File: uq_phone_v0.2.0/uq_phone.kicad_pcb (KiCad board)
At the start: 6 copper layers, 118.2 x 108 mm, 195 parts, among them J1 PJ-242C, J2 124018312112A, J3 BM03B-ACHSS-GAN-TF_LF__SN_, J4 20279-001E-03, J5 20279-001E-03, J6 Conn_ARM_SWD_TagConnect_TC2030, J8 MCS-302S-C1, M1 C08-00A, Q1 MMBT3904LP-7, Q2 MMBT3904LP-7, SW1 SKTAAAE010, SW10 SKTAAAE010, SW11 SKTAAAE010, SW12 SKTAAAE010, SW13 SKTAAAE010, SW14 SKTAAAE010, SW15 SKTAAAE010, SW16 SKSCLCE010, SW17 SKTAAAE010, SW18 SKTAAAE010, SW19 SKTAAAE010, SW2 SKTAAAE010, SW20 SKTAAAE010, SW21 SKTAAAE010, SW22 SKSCLCE010, SW23 SKTAAAE010, SW24 SKTAAAE010, SW25 SKTAAAE010, SW26 SKTAAAE010, SW27 SKTAAAE010, SW28 SKTAAAE010, SW29 SKTAAAE010, SW3 SKTAAAE010, SW30 SKTAAAE010, SW31 SKTAAAE010, SW32 SKTAAAE010, SW33 SKTAAAE010, SW34 SKTAAAE010, SW35 SKTAAAE010, SW36 SKTAAAE010, SW37 SKTAAAE010, SW38 SKTAAAE010, SW39 SKTAAAE010, SW4 SKTAAAE010, SW40 SKTAAAE010, SW41 SKTAAAE010, SW5 SKTAAAE010, SW6 SKSCLCE010, SW7 SKTAAAE010, SW8 SKTAAAE010, SW9 SKTAAAE010, U1 TPS62162DSGR, U10 TPD8F003DQDR, U11 LSM6DSVTR, U12 DRV2603RUNR, U13 TS3A5018RSVR, U14 NAU88C22YG, U15 TPS22964CYZPR, U2 MCP73871-2CCI_ML, U3 BQ27441DRZR-G1A, U4 WP SNAP-IN BASE_6000636, U5 TXB0108YZPR2, U6 STM32H733VGHx, U7 TXB0108YZPR2, U8 TPD3F303DQDR, U9 MCP1664T-E/OT

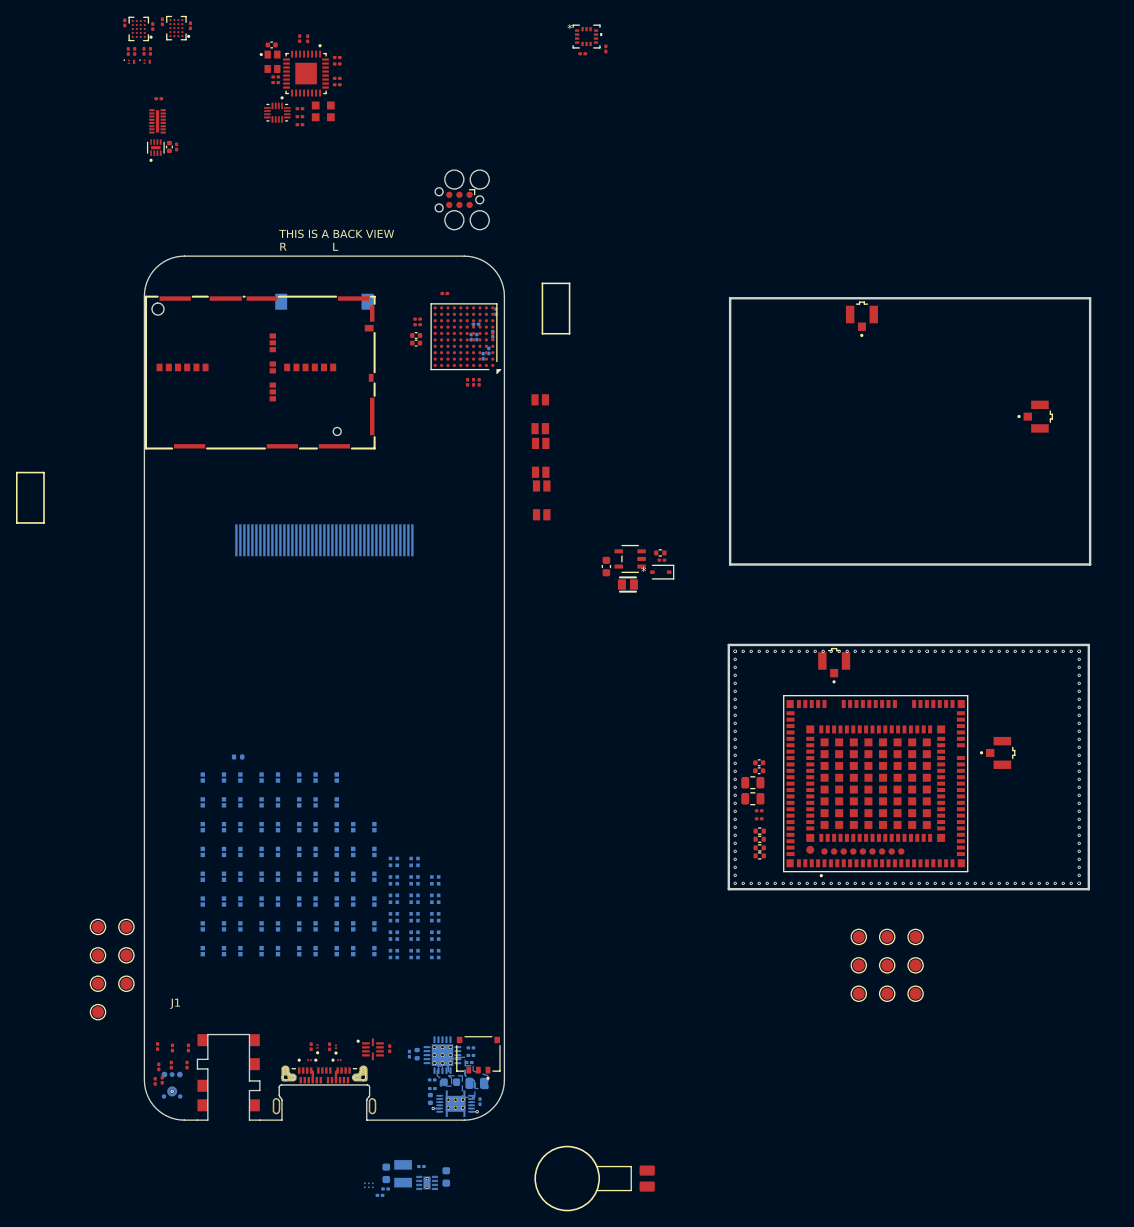
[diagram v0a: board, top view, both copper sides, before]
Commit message: New Layout
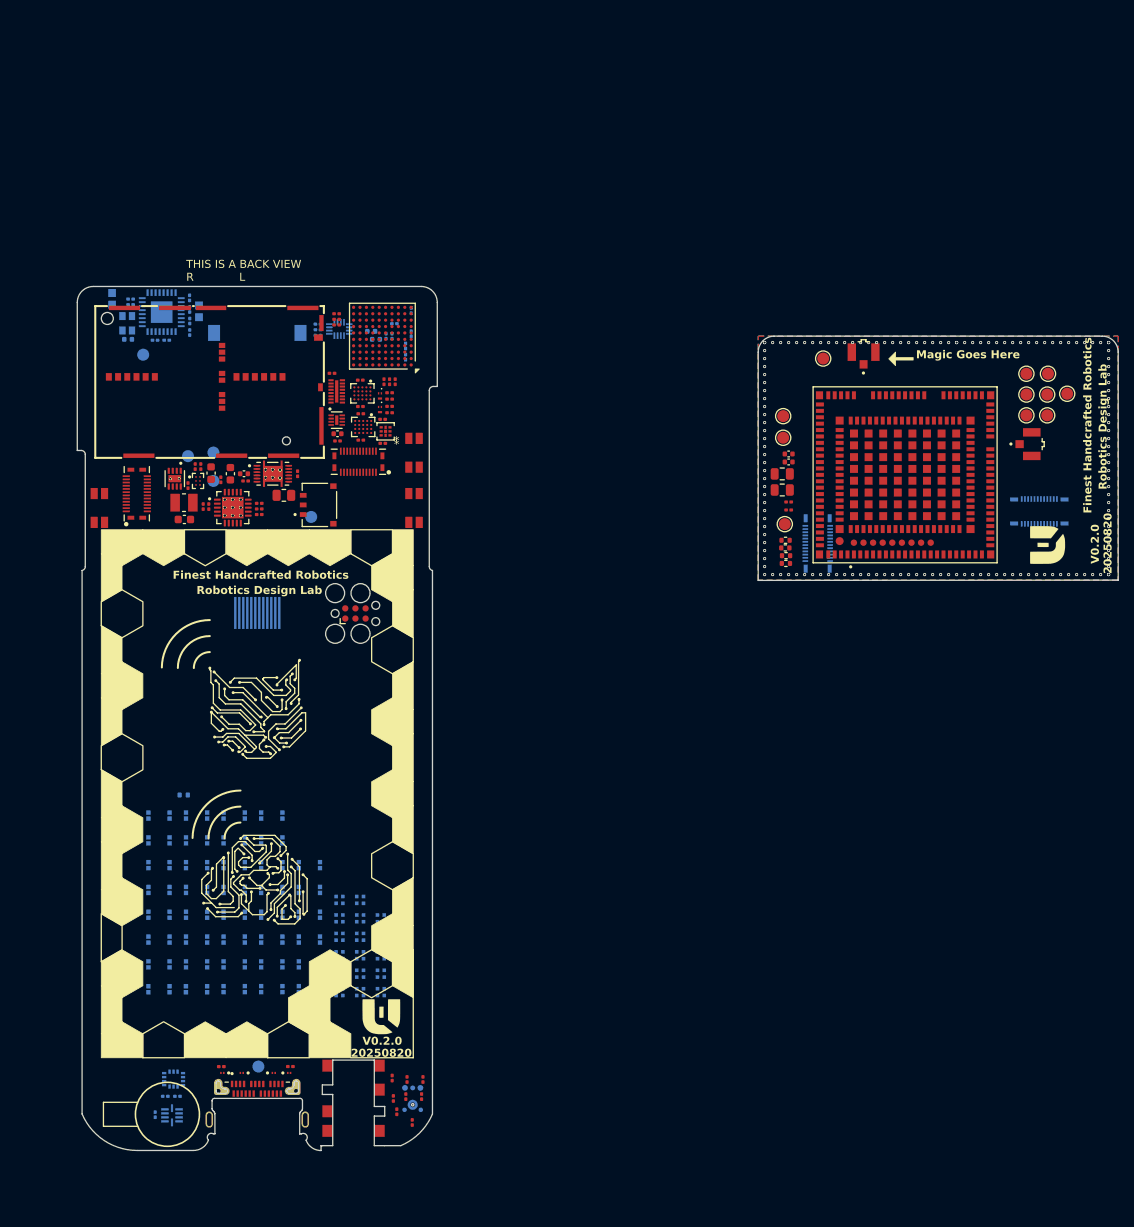
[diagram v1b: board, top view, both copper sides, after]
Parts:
- removed C27: 10uF, Capacitor_SMD:C_0603_1608Metric
- removed C28: 4.7uF, Capacitor_SMD:C_0201_0603Metric
- removed D2: PMEG2010EA, Diode_SMD:D_SOD-323
- removed Disp1: AFR240320A0-2.0INTM, custom_footprints:Display
- removed the J4 at (116.3, 24.4)
- removed the J5 at (138.6, 37.2)
- removed L2: 4.7uH, custom_footprints:IND-SMD_L2.0-W1.2_MTQH201208S4R7MBT
- removed R21: 4.7k, Resistor_SMD:R_0201_0603Metric
- removed R29: 3.83R, Resistor_SMD:R_0402_1005Metric
- removed U9: MCP1664T-E/OT, MCP1664T_E_OT:SOT-23-5_OT_MCH
- added C50: 100nF, Capacitor_SMD:C_0201_0603Metric, F.Cu at (56.4, 37.5)
- added C51: 100nF, Capacitor_SMD:C_0201_0603Metric, F.Cu at (56.5, 40.5)
- added DISP1: HS20HS072RX, custom_footprints:Display, B.Cu at (40.8, 53.9)
- added J10: 513382474, 513382474:CON_513382474, B.Cu at (138.5, 49.0)
- added J11: 513382474, 513382474:CON_513382474, B.Cu at (110.8, 53.0)
- added J7: 559092474, 559092474:CON_559092474, F.Cu at (25.7, 46.8)
- added J9: 559092474, 559092474:CON_559092474, F.Cu at (53.4, 42.8)
- added R4: 4.7k, Resistor_SMD:R_0201_0603Metric, F.Cu at (58.0, 32.8)
- added REF**: Art_large, custom_footprints:Art_large, F.Cu at (40.8, 84.3)
- added REF**: Art_small, custom_footprints:Art_small, F.Cu at (137.3, 40.5)
- added TP17: TestPoint, TestPoint:TestPoint_Pad_D1.5mm, F.Cu at (106.5, 39.8)
- added U16: TXB0108YZPR2, TXB0108YZPR2:YZP20, F.Cu at (53.9, 34.3)
- C1, C2, C3, C30, C31, C4, C5, C6, C7, L1, R1, R10, R11, R7, R8, R9, U1, U15, U2, U3: moved to F.Cu
- C25, C26, C29, C34, C35, C38, C39, C40, C41, C42, C43, C44, C45, C46, C47, FB1, FB2, OSC1, R32, R33, TP1, TP2, TP3, TP5, TP6, TP7, U11, U12, U13, U14: moved to B.Cu
- R5: footprint Resistor_SMD:R_0402_1005Metric -> Resistor_SMD:R_0201_0603Metric; moved to F.Cu
- U5: value TXB0108YZPR2 -> TCA9509MRVHR; footprint TXB0108YZPR2:YZP20 -> TCA9509MRVHR:RVH8_0P4X0P4
- moved C34 142.0 mm to (29.3, 122.1), turned to 0 degrees
- moved U11 140.2 mm to (30.3, 120.0), turned to 180 degrees
- moved C35 139.8 mm to (30.8, 122.1), turned to 180 degrees
- moved TP4 105.3 mm to (106.7, 50.6)
- moved C31 94.0 mm to (33.0, 43.4), turned to 90 degrees
- moved U1 93.5 mm to (30.4, 44.9), turned to -90 degrees
- moved C30 93.2 mm to (33.7, 43.4), turned to 90 degrees
- moved C1 92.8 mm to (35.0, 44.2)
- moved U15 90.6 mm to (33.4, 45.2), turned to 0 degrees
- moved R1 90.0 mm to (32.1, 45.8), turned to 90 degrees
- moved L1 88.2 mm to (31.6, 47.9), turned to 180 degrees
- moved C2 85.5 mm to (31.6, 50.0), turned to 0 degrees
- moved U3 82.0 mm to (42.7, 44.3)
- moved R8 81.7 mm to (45.8, 44.3), turned to 90 degrees
- moved C5 81.5 mm to (39.1, 44.3), turned to 180 degrees
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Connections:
- R22 pad 1: SDA -> SCL
- U4 pad 152: unconnected-(U4A-SAFE_PWR_REMOVE-Pad152) -> MOB_SAFE_PWR_REMOVE
- U4 pad 27: SIM_DATA -> SIM_CLK
- U4 pad 28: SIM_CLK -> SIM_DATA
- U7 pad A1: SCL -> unconnected-(U7-B2-PadA1)
- U7 pad A2: SDA -> unconnected-(U7-B1-PadA2)
- U7 pad A3: AUD_SDA -> unconnected-(U7-A1-PadA3)
- U7 pad A4: AUD_SCL -> unconnected-(U7-A2-PadA4)
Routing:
- net VUSB: track 2.57 -> 0.00 mm
- net SCL: track 0.83 -> 0.00 mm, vias 1 -> 0
- net FUEL_GPO: track 0.72 -> 0.00 mm, vias 1 -> 0
- removed copper zone on B.Cu, net Net-(U3-BAT)
- removed copper zone on B.Cu, net VBAT
- removed copper zone on B.Cu, net VUSB
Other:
- board size 118.2 x 108 mm -> 130.1 x 108 mm
- board text added: "SIM SOCKET"
- board text removed: "Socket Version"
